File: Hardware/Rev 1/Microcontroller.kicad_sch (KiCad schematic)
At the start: 23 parts, among them J1 Conn_01x04_Mae, J2 Conn_ARM_JTAG_SWD_10, J6 Conn_01x04_Mae, J7 Conn_01x04_Mae, J8 USB_C_Receptacle_USB2.0_14P, U2 STM32G474RETx, U4 MCP2542FDxMF, X2 ASCO

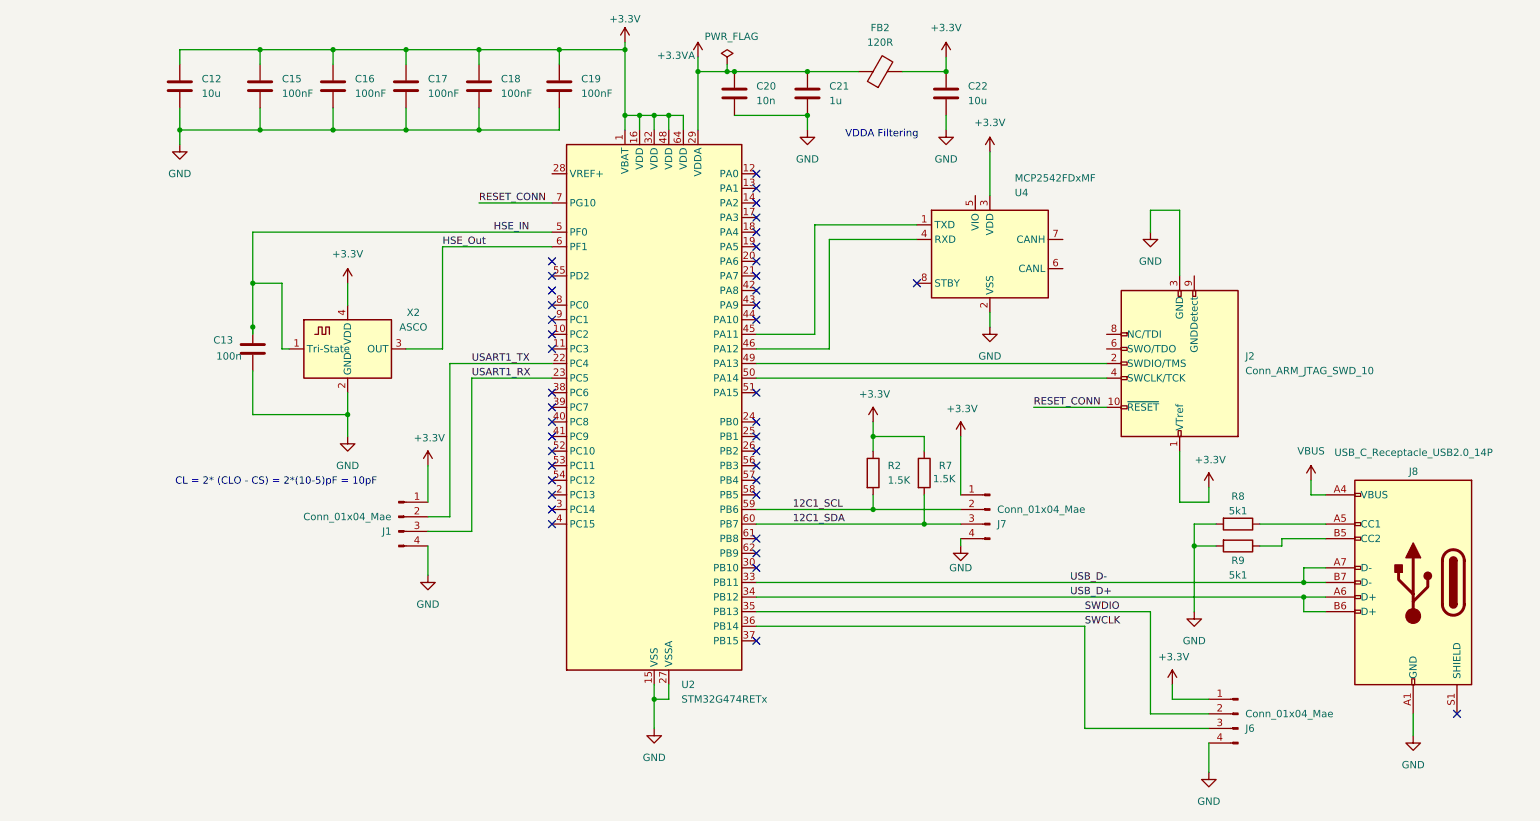
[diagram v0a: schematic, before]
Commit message: Done MCU Waiting review
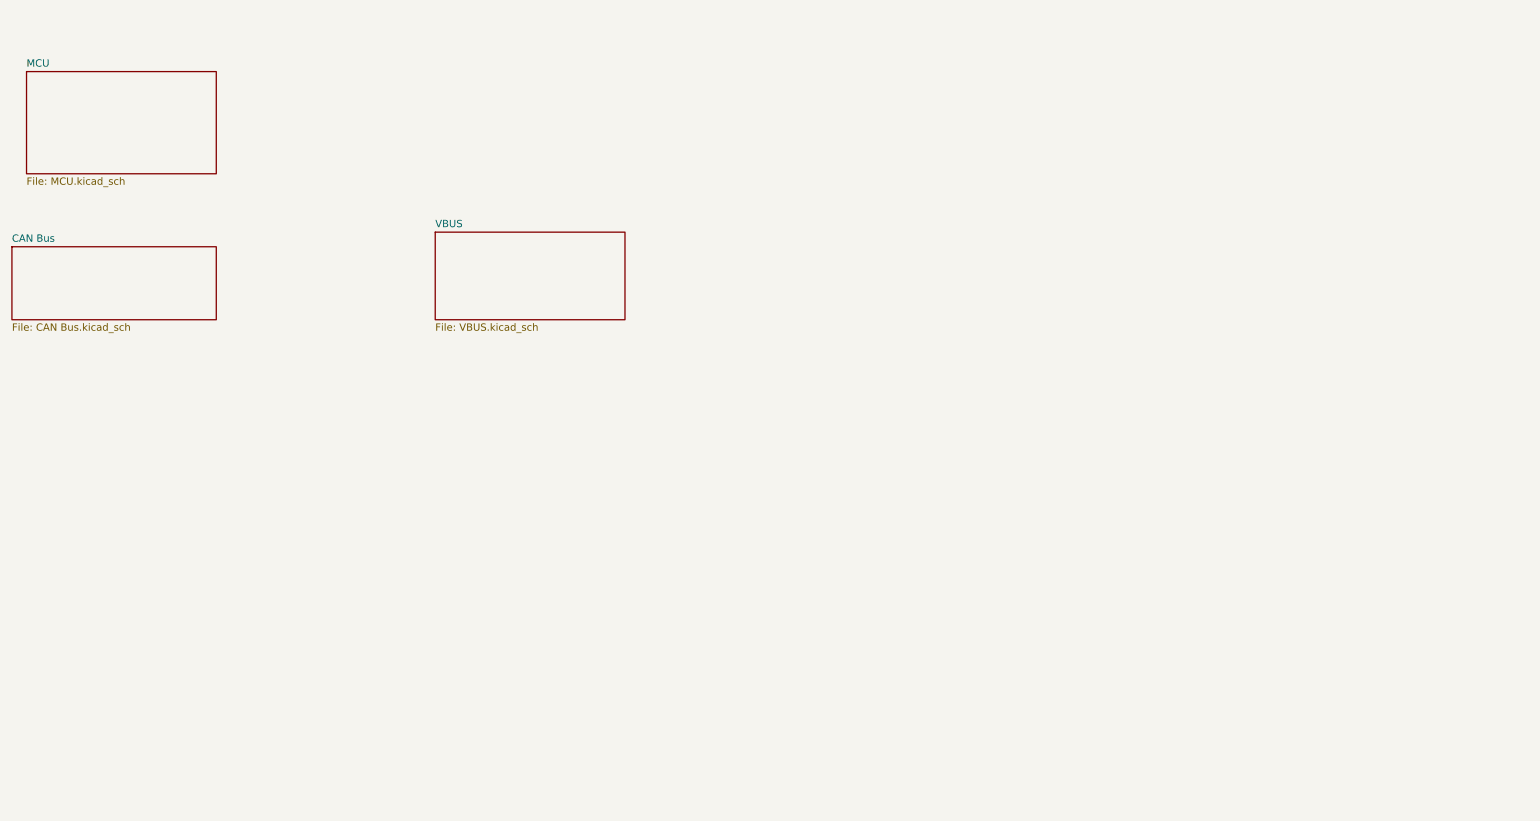
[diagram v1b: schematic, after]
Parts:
- removed C12: 10u, Capacitor_SMD:C_0603_1608Metric, symbol Device:C
- removed C13: 100n, Capacitor_SMD:C_0402_1005Metric, symbol Device:C
- removed C15, C16, C17, C18, C19: 100nF, Capacitor_SMD:C_0402_1005Metric, symbol Device:C
- removed C20: 10n, Capacitor_SMD:C_0603_1608Metric, symbol Device:C
- removed C21: 1u, Capacitor_SMD:C_0402_1005Metric, symbol Device:C
- removed C22: 10u, Capacitor_SMD:C_0402_1005Metric, symbol Device:C
- removed FB2: 120R, Inductor_SMD:L_0603_1608Metric, symbol Device:FerriteBead
- removed J1, J6, J7: Conn_01x04_Mae, Connector_PinHeader_2.54mm:PinHeader_1x04_P2.54mm_Vertical, symbol Connector:Conn_01x04_Pin
- removed J2: Conn_ARM_JTAG_SWD_10, symbol Connector:Conn_ARM_JTAG_SWD_10
- removed J8: USB_C_Receptacle_USB2.0_14P, symbol Connector:USB_C_Receptacle_USB2.0_14P
- removed R2, R7: 1.5K, Resistor_SMD:R_0402_1005Metric, symbol Device:R
- removed R8, R9: 5k1, symbol Device:R
- removed U2: STM32G474RETx, Package_QFP:LQFP-64_10x10mm_P0.5mm, symbol MCU_ST_STM32G4:STM32G474RETx
- removed U4: MCP2542FDxMF, Package_DFN_QFN:DFN-8-1EP_3x3mm_P0.65mm_EP1.55x2.4mm, symbol Interface_CAN_LIN:MCP2542FDxMF
- removed X2: ASCO, Oscillator:Oscillator_SMD_Abracon_ASCO-4Pin_1.6x1.2mm, symbol Oscillator:ASCO
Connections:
- no-connect marks 41 -> 0
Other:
- added sheet CAN Bus (CAN Bus.kicad_sch)
- added sheet MCU (MCU.kicad_sch)
- added sheet VBUS (VBUS.kicad_sch)
- note removed: "CL = 2* (CLO - CS) = 2*(10-5)pF = 10pF"
- note removed: "VDDA Filtering"
